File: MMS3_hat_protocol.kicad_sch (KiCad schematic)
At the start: 26 parts, among them J12 Conn_01x04_Pin, J13 Conn_01x04_Pin, J4 Conn_01x04_Pin, J6 Conn_01x04_Pin, J9 Conn_01x04_Pin, U13 PCA9306, U3 AMS1117, U6 TCA9535PWR

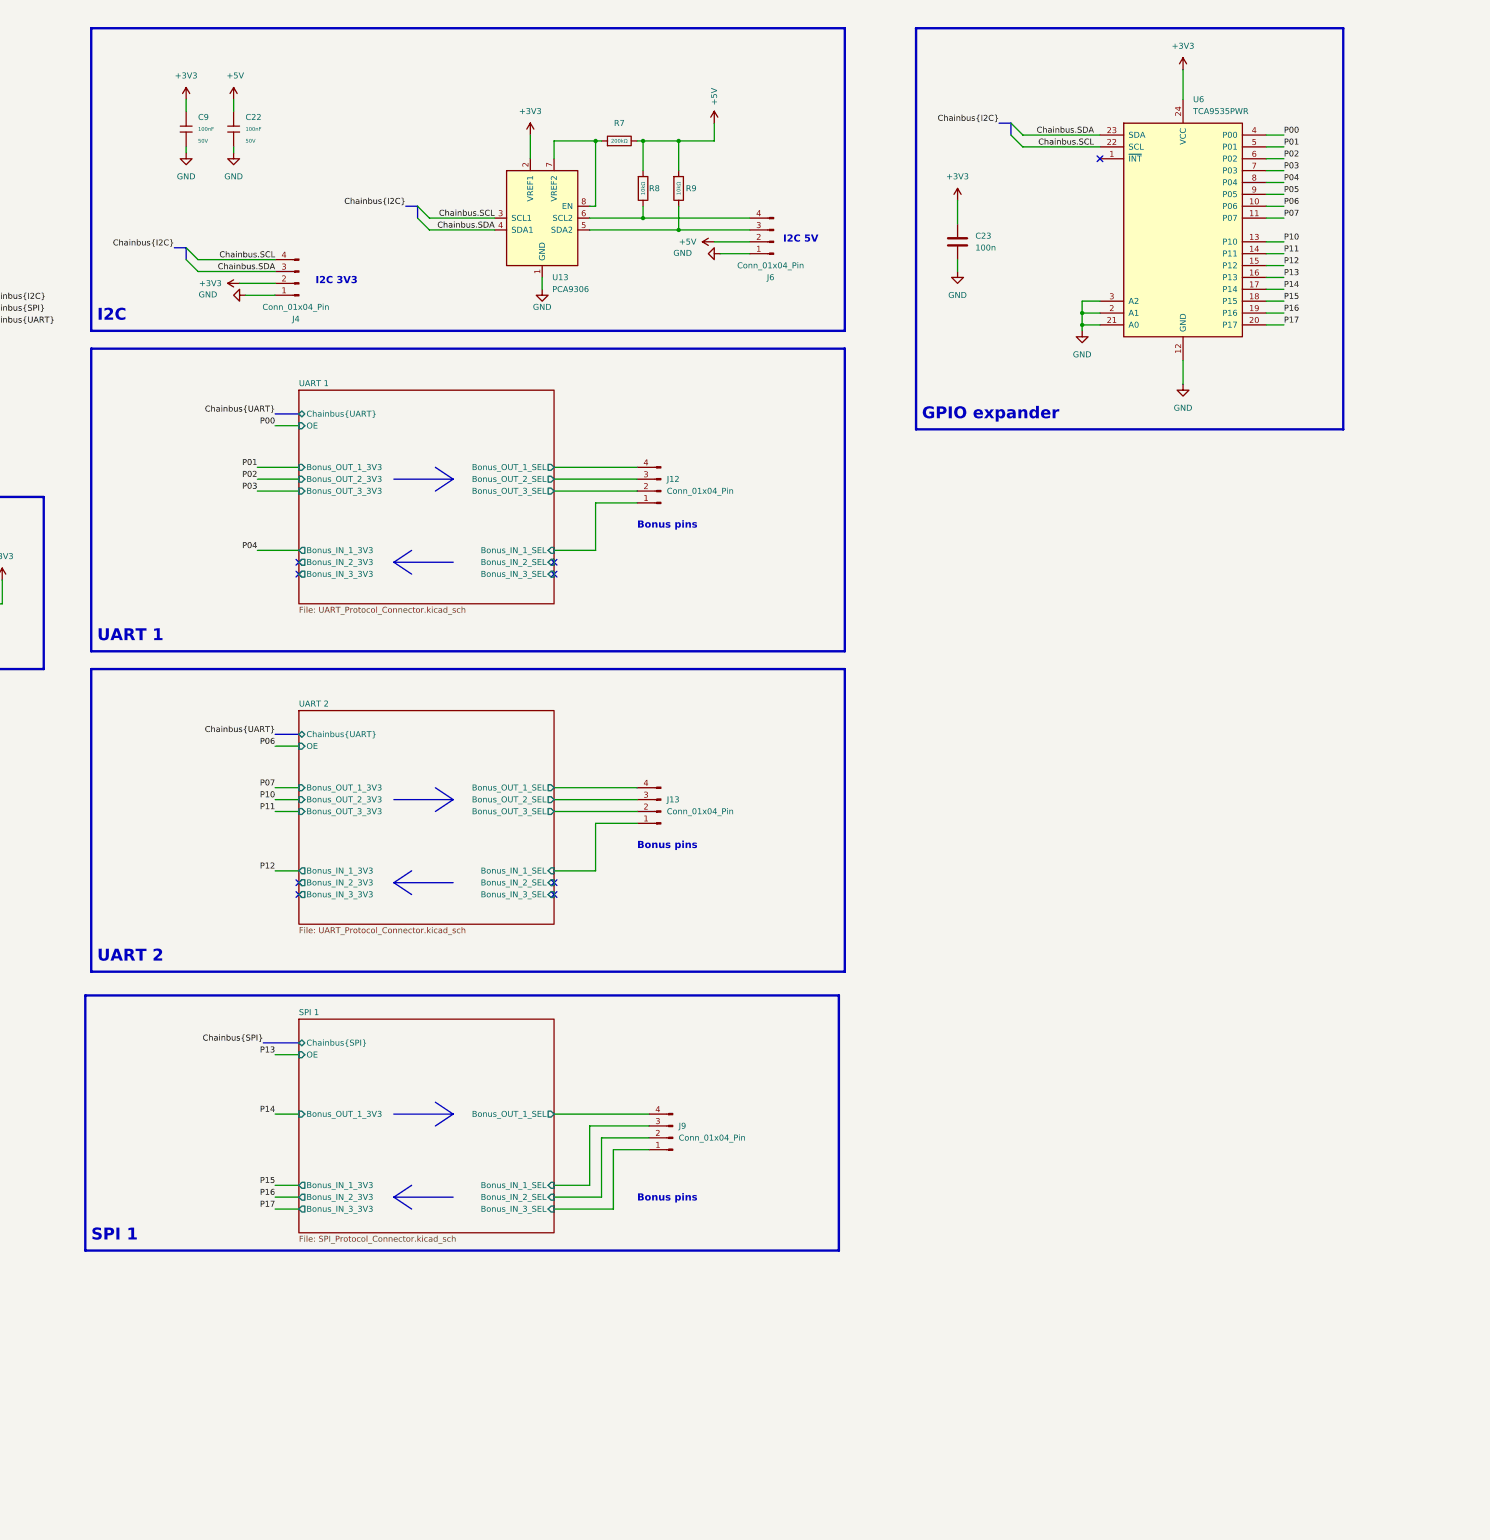
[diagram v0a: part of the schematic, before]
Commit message: finished schematic
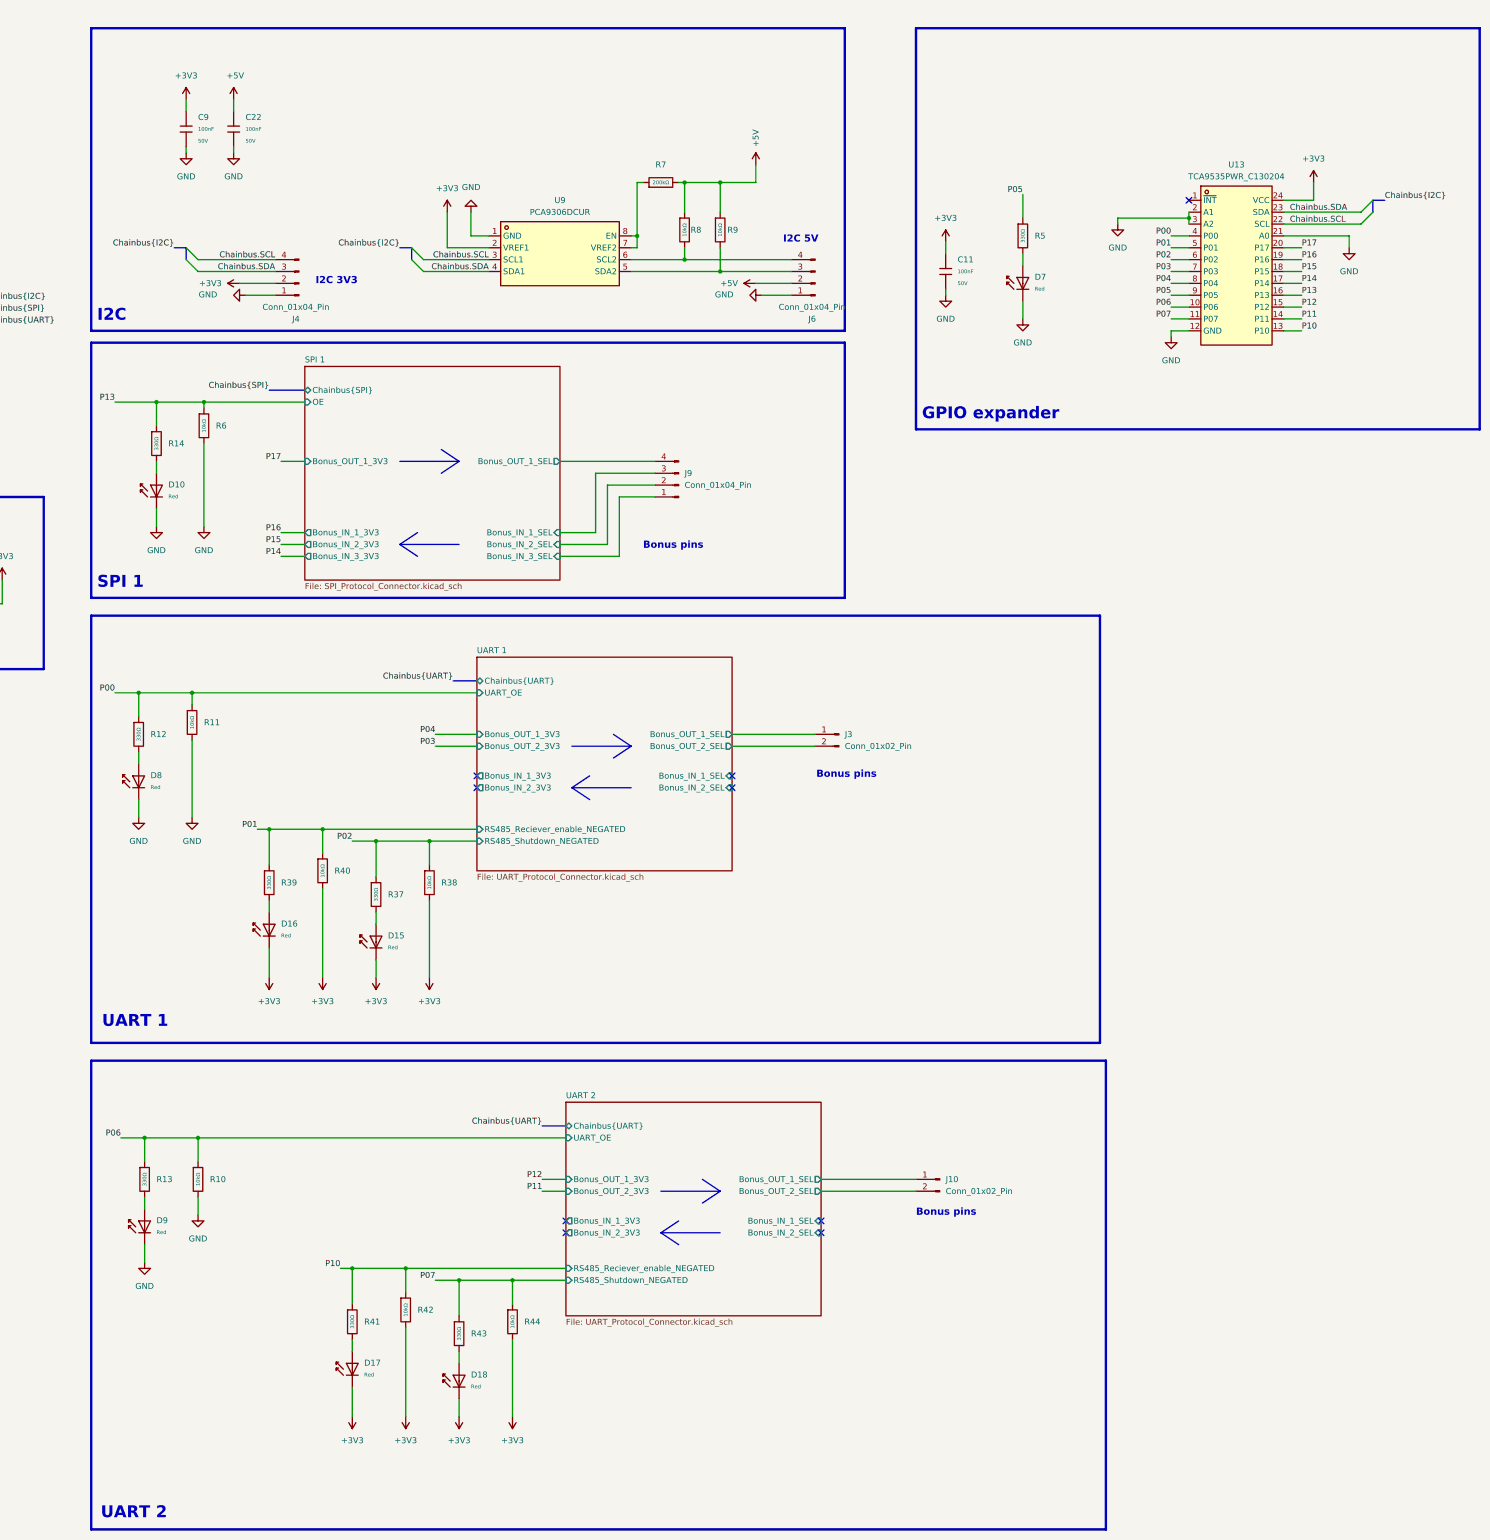
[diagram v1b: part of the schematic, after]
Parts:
- removed C23: 100n, PCM_JLCPCB:C_0603, symbol Device:C
- removed J12, J13: Conn_01x04_Pin, Connector_JST:JST_XH_S4B-XH-A_1x04_P2.50mm_Horizontal, symbol Connector:Conn_01x04_Pin
- removed U13: PCA9306, Package_SO:VSSOP-8_2.3x2mm_P0.5mm, symbol Interface:PCA9306
- removed U6: TCA9535PWR, Package_SO:TSSOP-24_4.4x7.8mm_P0.65mm, symbol Interface_Expansion:TCA9535PWR
- added C11: 100nF, PCM_JLCPCB:C_0603, symbol PCM_JLCPCB-Capacitors:0603,100nF
- added D10, D15, D16, D17, D18, D7, D8, D9: Red, PCM_JLCPCB:D_0603, symbol PCM_JLCPCB-Diodes:LED,0603,Red
- added J10, J3: Conn_01x02_Pin, Connector_PinSocket_2.54mm:PinSocket_1x02_P2.54mm_Vertical, symbol Connector:Conn_01x02_Pin
- added R10, R11, R38, R40, R42, R44, R6: 10kΩ, PCM_JLCPCB:R_0402, symbol PCM_JLCPCB-Resistors:0402,10kΩ
- added R12, R13, R14, R37, R39, R41, R43, R5: 330Ω, PCM_JLCPCB:R_0402, symbol PCM_JLCPCB-Resistors:0402,330Ω
- added U13: TCA9535PWR_C130204, TCA9535PWR:TSSOP-24_L7.8-W4.4-P0.65-LS6.4-BL, symbol TCA9535PWR_test:TCA9535PWR_C130204
- added U9: PCA9306DCUR, PCA9306DCUR:SSOP-8_L2.0-W2.3-P0.50-LS3.1-BR, symbol PCA9306DCUR:PCA9306DCUR
- H7, H8, H9, PN1: value ~ -> (none)
- J9: footprint Connector_JST:JST_XH_S4B-XH-A_1x04_P2.50mm_Horizontal -> Connector_PinSocket_2.54mm:PinSocket_1x04_P2.54mm_Vertical
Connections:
- net +3V3: now also C11.1, D15.1, D16.1, D17.1, D18.1, R38.2, R40.2, R42.2, R44.2, U13.24 (VCC), U9.2 (VREF1)
- net Chainbus.SCL: now also U13.22 (SCL), U9.3 (SCL1)
- net Chainbus.SDA: now also U13.23 (SDA), U9.4 (SDA1)
- net GND: now also C11.2, D10.1, D7.1, D8.1, D9.1, R10.2, R11.2, R6.2, U13.12 (GND), U13.2 (A1), U13.21 (A0), U13.3 (A2), U9.1 (GND)
- net P00: now also R11.1, R12.1, U13.4 (P00)
- net P01: now also R39.1, R40.1, U13.5 (P01)
- net P02: now also R37.1, R38.1, U13.6 (P02)
- net P03: now also U13.7 (P03)
- net P04: now also U13.8 (P04)
- net P05: now also R5.1, U13.9 (P05)
- net P06: now also R10.1, R13.1, U13.10 (P06)
- net P07: now also R43.1, R44.1, U13.11 (P07)
- net P10: now also R41.1, R42.1, U13.13 (P10)
- net P11: now also U13.14 (P11)
- net P12: now also U13.15 (P12)
- net P13: now also R14.1, R6.1, U13.16 (P13)
- net P14: now also U13.17 (P14)
- net P15: now also U13.18 (P15)
- net P16: now also U13.19 (P16)
- net P17: now also U13.20 (P17)
- net UART 1/Bonus_OUT_1_SEL: now also J3.1 (Pin_1)
- net UART 1/Bonus_OUT_2_SEL: now also J3.2 (Pin_2)
- net UART 2/Bonus_OUT_1_SEL: now also J10.1 (Pin_1)
- net UART 2/Bonus_OUT_2_SEL: now also J10.2 (Pin_2)
- net at J6.3 (Pin_3), R9.2: now also U9.5 (SDA2)
- net at J6.4 (Pin_4), R8.2: now also U9.6 (SCL2)
- net at R7.1: now also U9.7 (VREF2), U9.8 (EN)
- new net: D8.2, R12.2
- new net: D10.2, R14.2
- new net: D9.2, R13.2
- new net: D15.2, R37.2
- new net: D7.2, R5.2
- new net: D16.2, R39.2
- new net: D18.2, R43.2
- new net: D17.2, R41.2
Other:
- sheet UART 1 ports: added RS485_Reciever_enable_NEGATED, RS485_Shutdown_NEGATED, UART_OE; removed Bonus_IN_3_3V3, Bonus_IN_3_SEL, Bonus_OUT_3_3V3, Bonus_OUT_3_SEL, OE
- sheet UART 2 ports: added RS485_Reciever_enable_NEGATED, RS485_Shutdown_NEGATED, UART_OE; removed Bonus_IN_3_3V3, Bonus_IN_3_SEL, Bonus_OUT_3_3V3, Bonus_OUT_3_SEL, OE
- moved on the sheet: J9
